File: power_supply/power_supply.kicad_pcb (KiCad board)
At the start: 2 copper layers, 100 x 50 mm, 12 parts, among them J1 Input, J2 Input

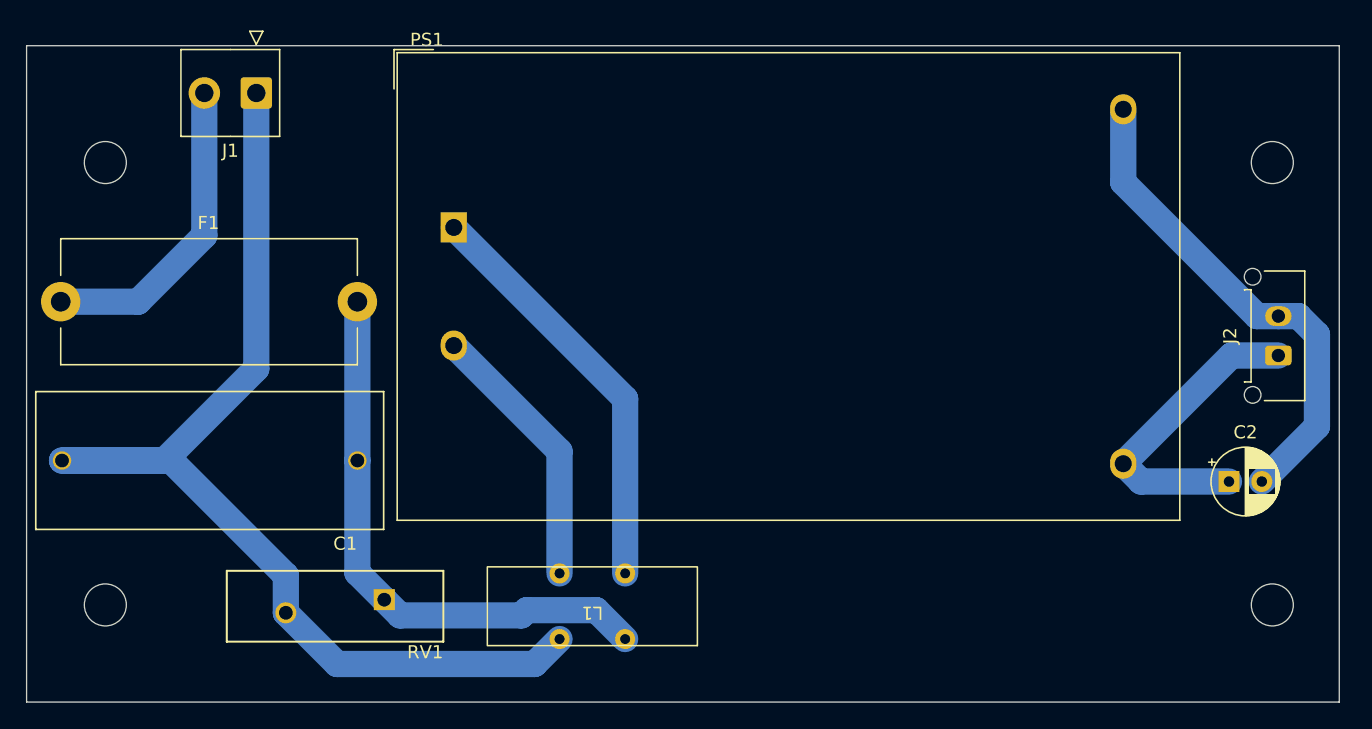
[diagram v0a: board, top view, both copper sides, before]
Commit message: upd
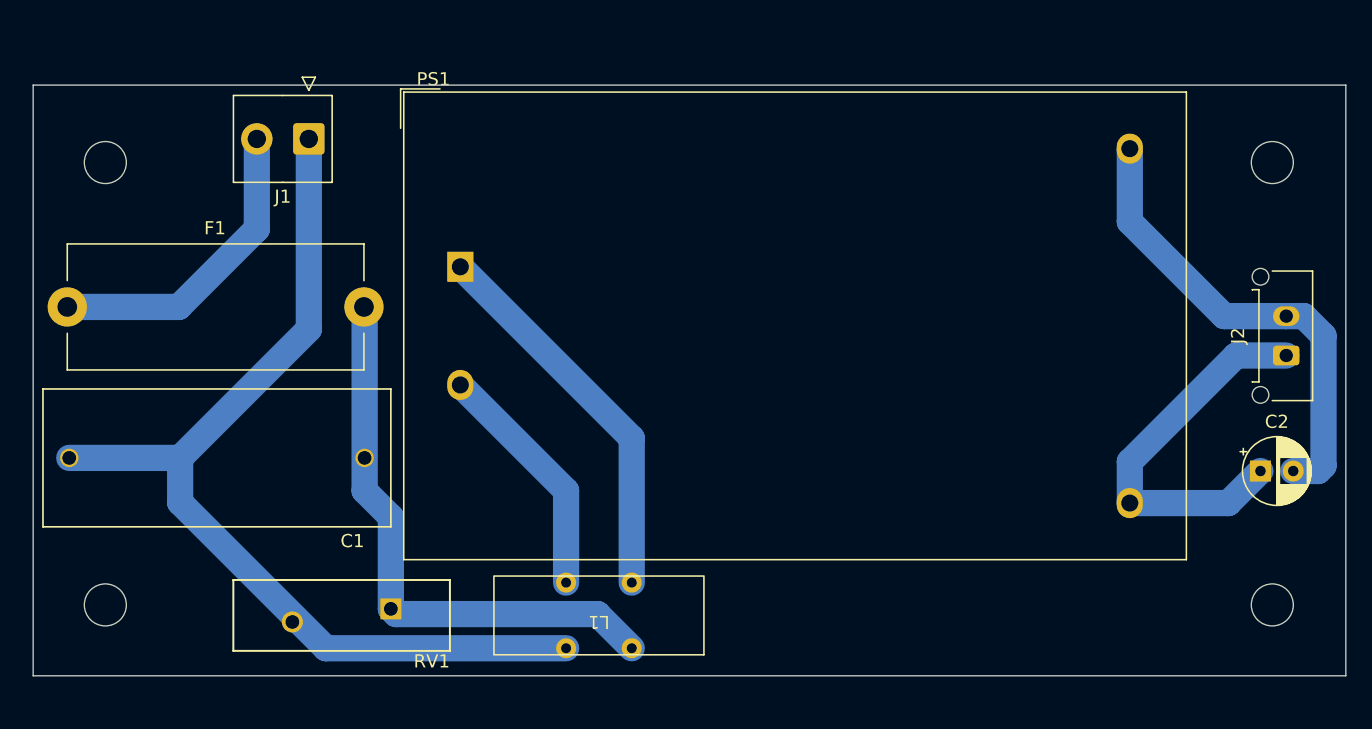
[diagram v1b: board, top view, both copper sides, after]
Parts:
- moved J1 5.32 mm to (111.0, 60.1)
- moved PS1 3.04 mm to (122.5, 69.8)
- moved C2 2.52 mm to (183.4, 85.4)
- moved L1 0.86 mm to (133.1, 96.4)
- moved RV1 0.86 mm to (113.5, 96.4)
- moved F1 0.64 mm to (92.5, 72.9)
- moved J2 0.60 mm to (185.4, 76.6)
- moved C1 0.59 mm to (104.0, 84.4)
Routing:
- net Net-(J1-Pin_1): track 85.5 -> 73.9 mm
- net Net-(J2-Pin_1): track 23.9 -> 29.4 mm
- net Net-(PS1-AC/N): track 20.7 -> 18.4 mm
- net Net-(PS1-AC/L): track 31.8 -> 29.5 mm
- net Net-(J2-Pin_2): track 38.1 -> 36.3 mm
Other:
- board size 100 x 50 mm -> 100 x 45 mm
